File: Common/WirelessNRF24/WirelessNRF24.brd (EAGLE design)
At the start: 100 x 80 mm, 16 parts, among them U1 NRF24L01ALT1, Y1 ANTENNA2SMD5, Y2 16MHz

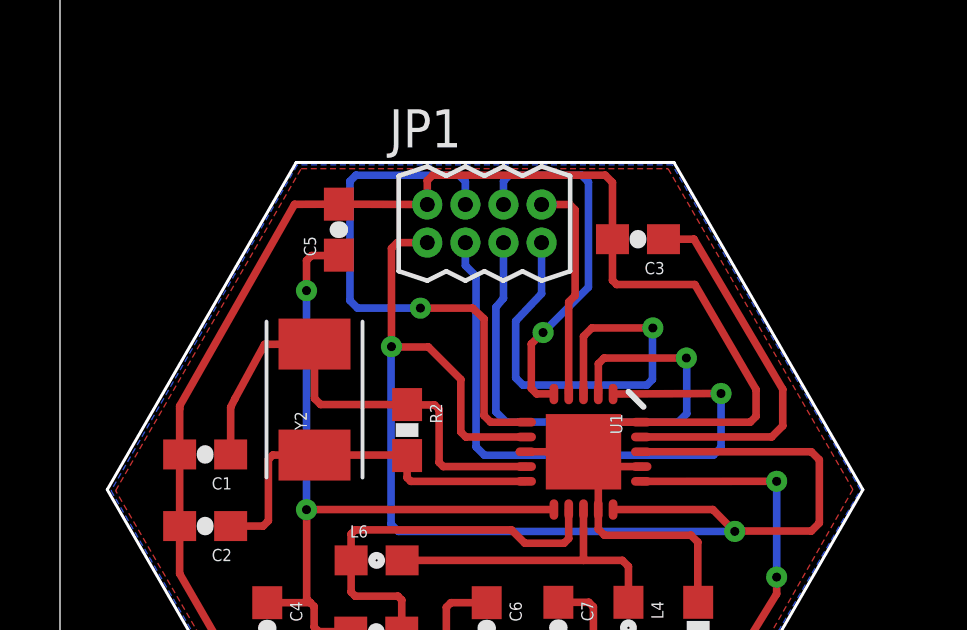
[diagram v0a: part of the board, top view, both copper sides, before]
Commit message: another round of minor fixes
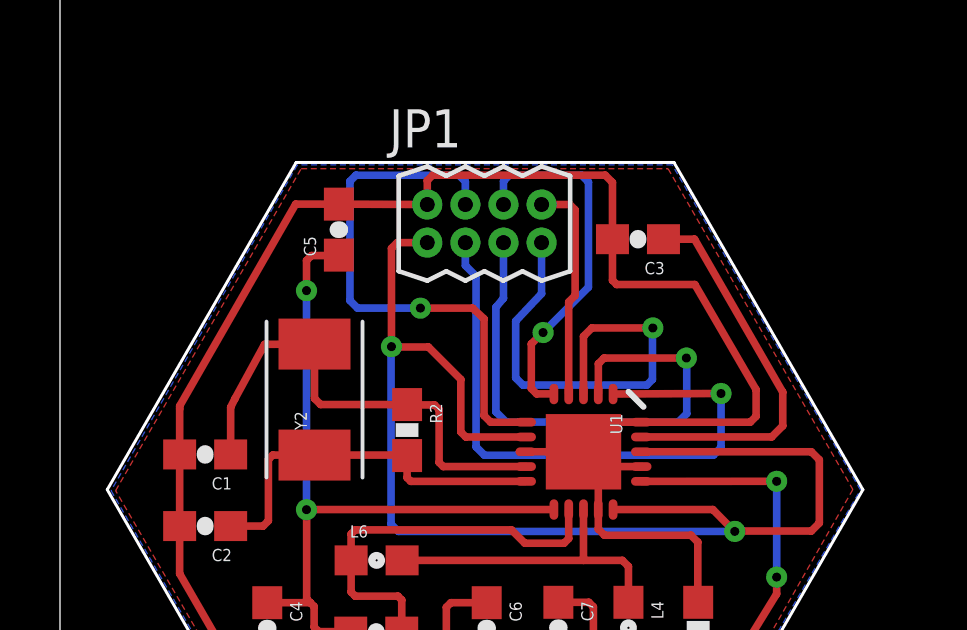
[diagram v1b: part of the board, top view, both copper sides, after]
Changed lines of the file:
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@@
 <wire x1="3.9887" y1="13.6271" x2="3.9887" y2="15.1467" width="0.254" layer="1"/>
 <wire x1="3.9887" y1="15.1467" x2="3.9878" y2="15.24" width="0.254" layer="1"/>
-<wire x1="3.9878" y1="15.24" x2="7.8173" y2="21.9647" width="0.254" layer="1"/>
-<wire x1="7.8173" y1="21.9647" x2="9.2964" y2="21.9701" width="0.254" layer="1"/>
+<wire x1="3.9878" y1="15.24" x2="7.8551" y2="21.971" width="0.254" layer="1"/>
+<wire x1="7.8551" y1="21.971" x2="9.2964" y2="21.9701" width="0.254" layer="1"/>
 <wire x1="6.9215" y1="7.1882" x2="5.4102" y2="7.1882" width="0.254" layer="1"/>
 <wire x1="5.4102" y1="7.1882" x2="3.9878" y2="9.652" width="0.254" layer="1"/>
@@
 <contactref element="C3" pad="1"/>
 <contactref element="U1" pad="19"/>
-<wire x1="20.1159" y1="20.8026" x2="21.1328" y2="20.8026" width="0.254" layer="1"/>
-<wire x1="21.1328" y1="20.8026" x2="24.0919" y2="15.7988" width="0.254" layer="1"/>
-<wire x1="24.0919" y1="15.7988" x2="24.0919" y2="14.5796" width="0.254" layer="1"/>
+<wire x1="20.1159" y1="20.8026" x2="21.1517" y2="20.8026" width="0.254" layer="1"/>
+<wire x1="21.1517" y1="20.8026" x2="24.0919" y2="15.7043" width="0.254" layer="1"/>
+<wire x1="24.0919" y1="15.7043" x2="24.0919" y2="14.5796" width="0.254" layer="1"/>
 <wire x1="24.0919" y1="14.5796" x2="23.7236" y2="14.2113" width="0.254" layer="1"/>
 <wire x1="23.7236" y1="14.2113" x2="19.3773" y2="14.2113" width="0.254" layer="1"/>

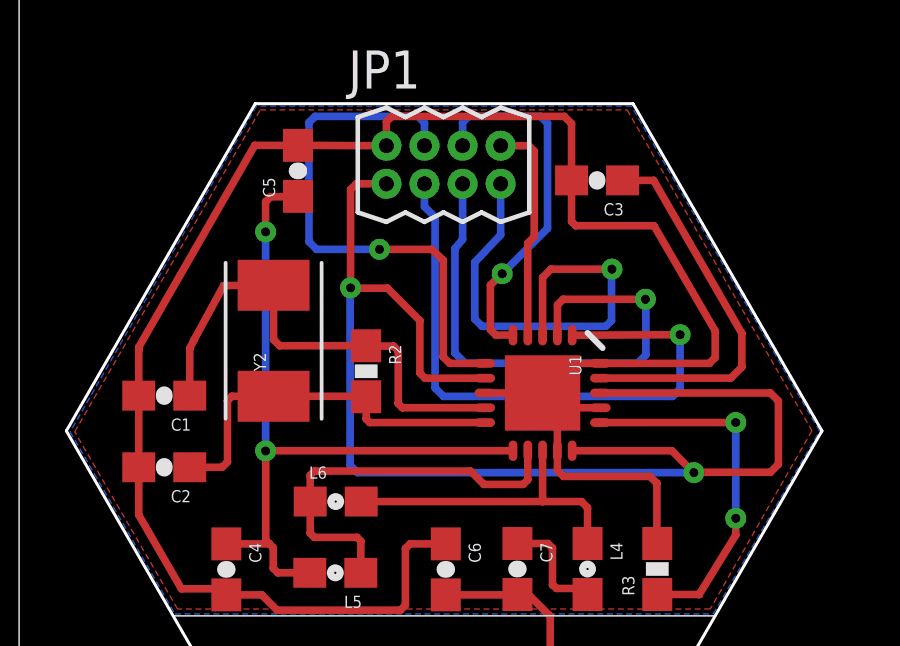
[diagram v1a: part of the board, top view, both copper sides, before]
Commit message: unknown changes! :(
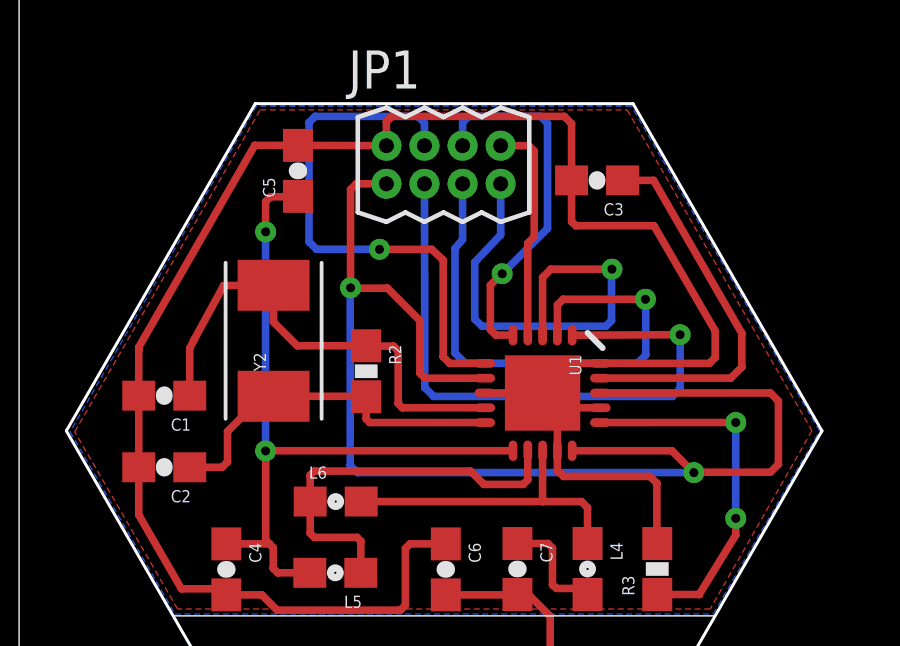
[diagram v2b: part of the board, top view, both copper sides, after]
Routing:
- net N$2: track 12.8 -> 12.1 mm
